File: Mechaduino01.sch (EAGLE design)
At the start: 61 parts, among them IC1 SAMD21G18A-AUT, Q2 NFET, Q3 BSS138, Q4 BSS138, Q5 BSS138, U1 TLV70233PDBVR, Y1 32,768Khz

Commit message: moved things around
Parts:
- D1: device MF_Discrete_Semiconductor:DIODE_SMA -> MF_Discrete_Semiconductor:DIODE_SOD-123
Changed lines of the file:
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@@
 <part name="R11" library="adafruit" deviceset="R-US_" device="R0402-VISHAY" value="10K"/>
 <part name="U1" library="MF_IC_Power" deviceset="TLV702" device="33PDBVR"/>
-<part name="D1" library="MF_Discrete_Semiconductor" deviceset="DIODE" device="_SMA"/>
+<part name="D1" library="MF_Discrete_Semiconductor" deviceset="DIODE" device="_SOD-123"/>
 </parts>
 <sheets>

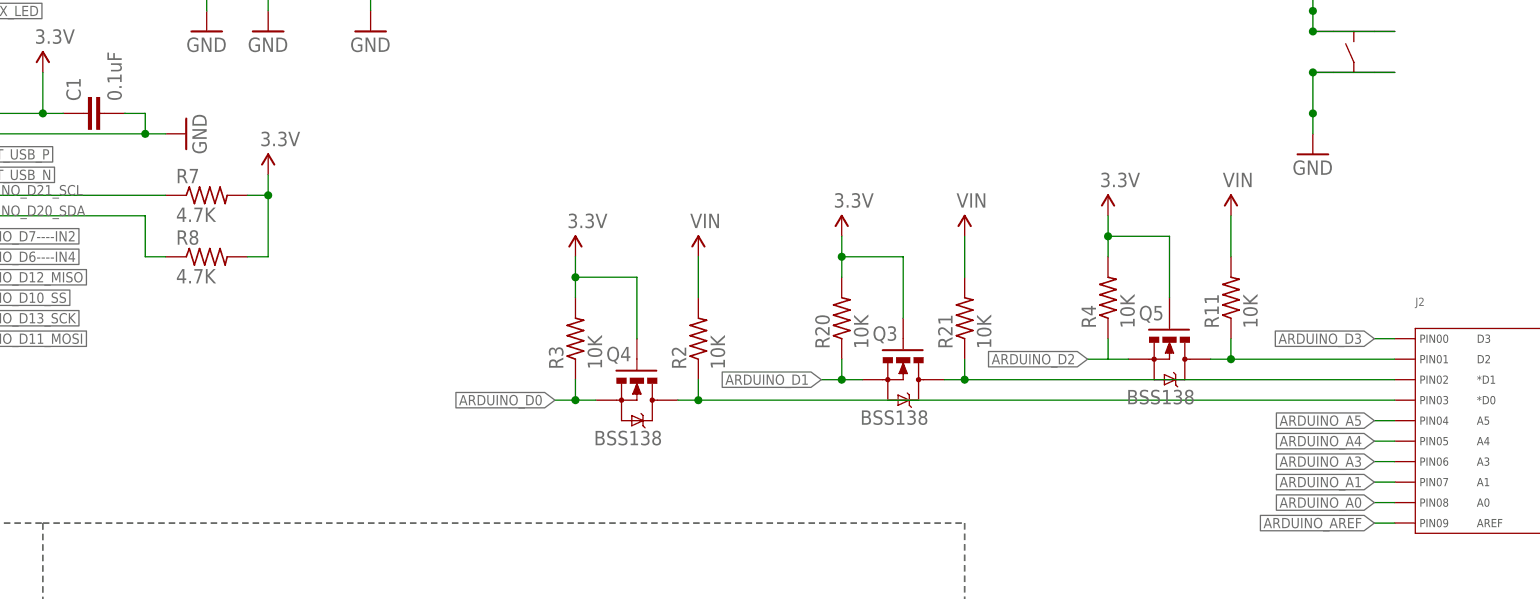
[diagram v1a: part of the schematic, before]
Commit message: commit after rollback issues
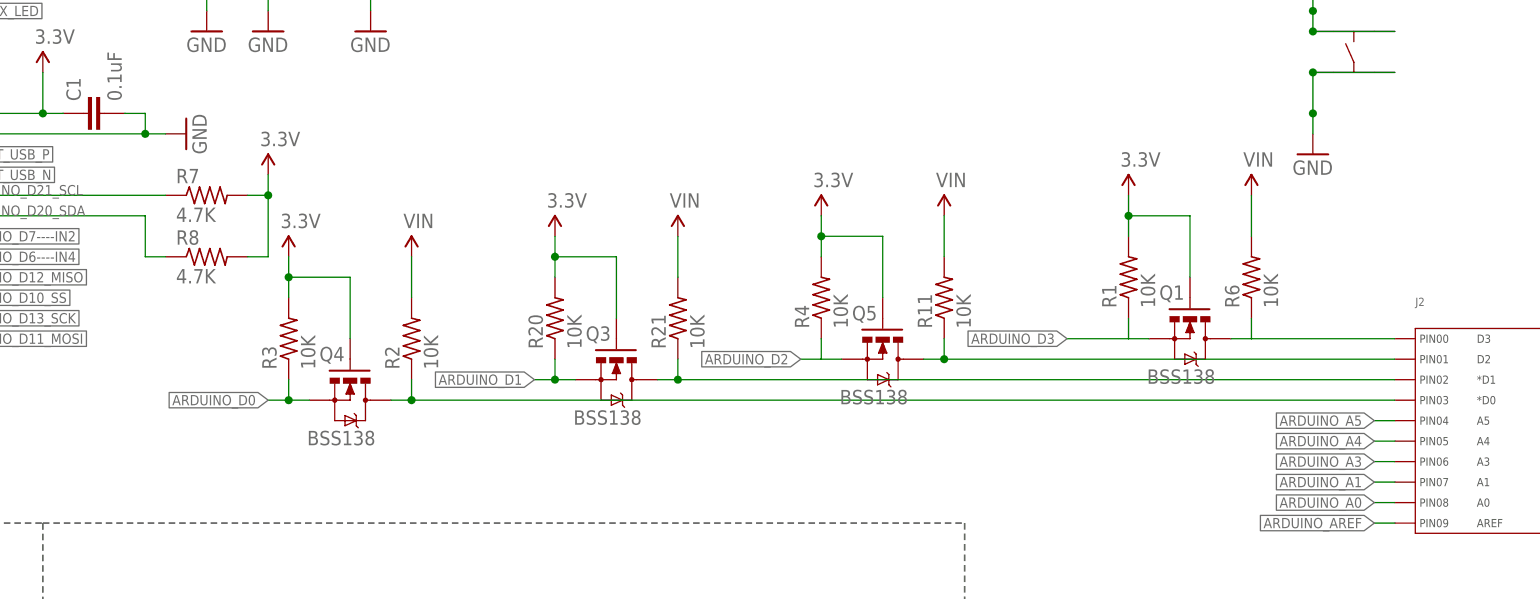
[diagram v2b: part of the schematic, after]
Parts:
- added Q1: BSS138, SparkFun:MOSFET-NCHANNELSMD
- added R1, R6: 10K, adafruit:R-US_R0402-VISHAY
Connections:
- new net HV4: J2.PIN0, Q1.D, R6.1
- net 3.3V: now also Q1.G, R1.2
- net ARDUINO_D3: now also Q1.S, R1.1; no longer J2.PIN0
- net VIN: now also R6.2
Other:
- moved on the sheet: Q3, Q4, Q5, R11, R2, R20, R21, R3, R4
